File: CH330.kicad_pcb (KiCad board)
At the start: 2 copper layers, 10 x 10 mm, 9 parts, among them J1 USB_B_Micro, J2 Conn_01x04_Female, U1 CH330

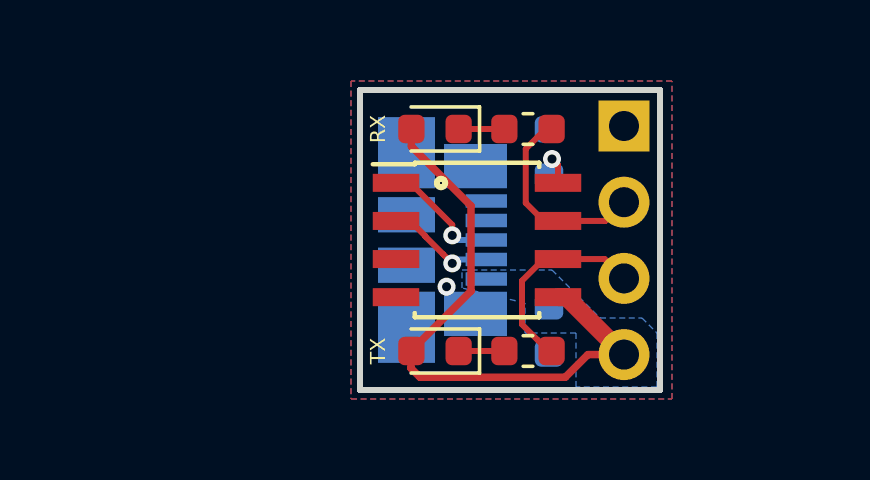
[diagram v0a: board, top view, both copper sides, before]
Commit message: add: pcb layout
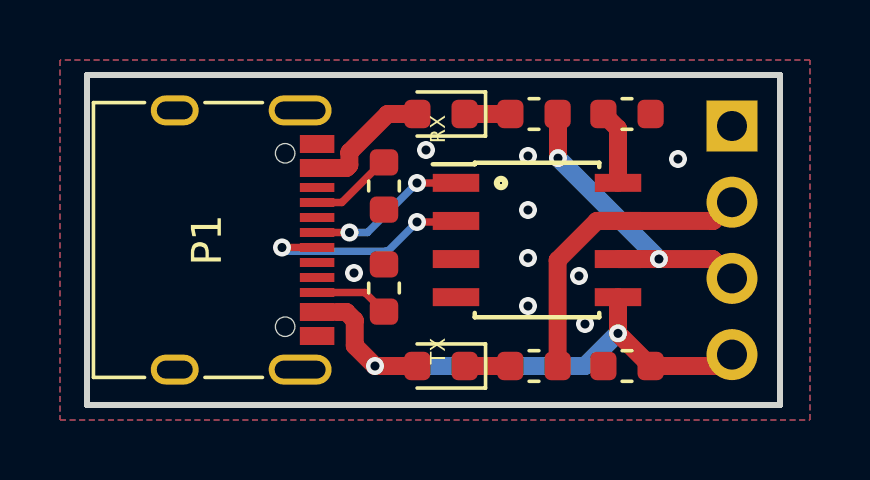
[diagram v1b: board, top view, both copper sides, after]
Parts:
- removed J1: USB_B_Micro, Connector_USB:USB_Micro-B_Molex_47346-0001
- added P1: USB_C_Plug_USB2.0, Connector_USB:USB_C_Receptacle_XKB_U262-16XN-4BVC11, F.Cu at (179.9, 80.0)
- added R3: 5.1k, Resistor_SMD:R_0603_1608Metric, F.Cu at (185.8, 78.2)
- added R4: 5.1k, Resistor_SMD:R_0603_1608Metric, F.Cu at (185.8, 81.6)
- C1, C2: moved to F.Cu
- J2: footprint otter:PinHeader_1x04_P2.54mm_Vertica_WITHOUT_SILK -> Connector_PinHeader_2.54mm:PinHeader_1x04_P2.54mm_Vertical
- U1: value CH330 -> CH330N
- moved J2 3.60 mm to (197.4, 76.2)
- moved C2 2.91 mm to (193.9, 75.8), turned to 0 degrees
- moved C1 2.86 mm to (193.9, 84.2), turned to 180 degrees
- moved U1 2.00 mm to (190.9, 80.0)
- moved R1 0.54 mm to (190.8, 84.2)
- moved R2 0.54 mm to (190.8, 75.8)
- moved D1 0.54 mm to (187.7, 84.2)
- moved D2 0.54 mm to (187.7, 75.8)
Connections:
- net /V3 renamed Net-(C2-Pad1)
- J2 pad 2: /RXD -> Net-(J2-Pad2)
- J2 pad 3: /TXD -> Net-(J2-Pad3)
- R1 pad 2: /TXD -> Net-(J2-Pad2)
- R2 pad 2: /RXD -> Net-(J2-Pad3)
- U1 pad 1: /D+ -> Net-(P1-PadA6)
- U1 pad 2: /D- -> Net-(P1-PadA7)
- U1 pad 4: /RTS -> (no net)
- U1 pad 6: /TXD -> Net-(J2-Pad3)
- U1 pad 7: /RXD -> Net-(J2-Pad2)
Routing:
- net Net-(J2-Pad3): track 0.00 -> 10.3 mm, vias 0 -> 2
- net Net-(J2-Pad2): track 0.00 -> 10.1 mm
- net Net-(P1-PadA7): track 0.00 -> 7.44 mm, vias 0 -> 2
- net /TXD: track 6.82 -> 0.00 mm
- net /RXD: track 6.80 -> 0.00 mm
- net Net-(P1-PadA6): track 0.00 -> 5.32 mm, vias 0 -> 2
- net /D+: track 4.00 -> 0.00 mm, vias 1 -> 0
- net /D-: track 3.66 -> 0.00 mm, vias 1 -> 0
- net VBUS: track 20.2 -> 23.3 mm, vias 0 -> 2
- net Net-(P1-PadA5): track 0.00 -> 2.78 mm
- net Net-(P1-PadB5): track 0.00 -> 2.49 mm
- net Net-(C2-Pad1): track 1.51 -> 2.50 mm, vias 1 -> 0
- net GND: vias 1 -> 9
- removed copper zone on B.Cu, net VBUS
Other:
- board size 10 x 10 mm -> 23.1 x 11 mm
